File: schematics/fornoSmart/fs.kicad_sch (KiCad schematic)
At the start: 7 parts, among them J1 display, J2 rtc, J3-B rele, J4 speaker, J5 led, J6 VIN-12V

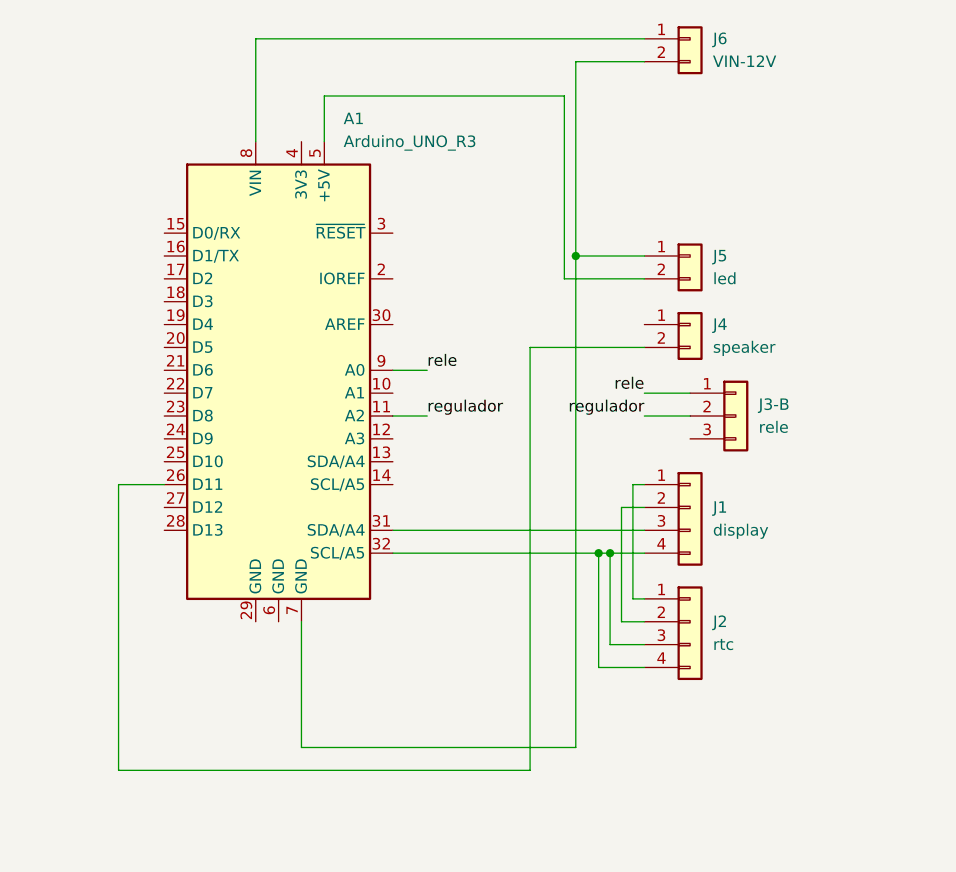
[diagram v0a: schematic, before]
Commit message: 2025-12 update
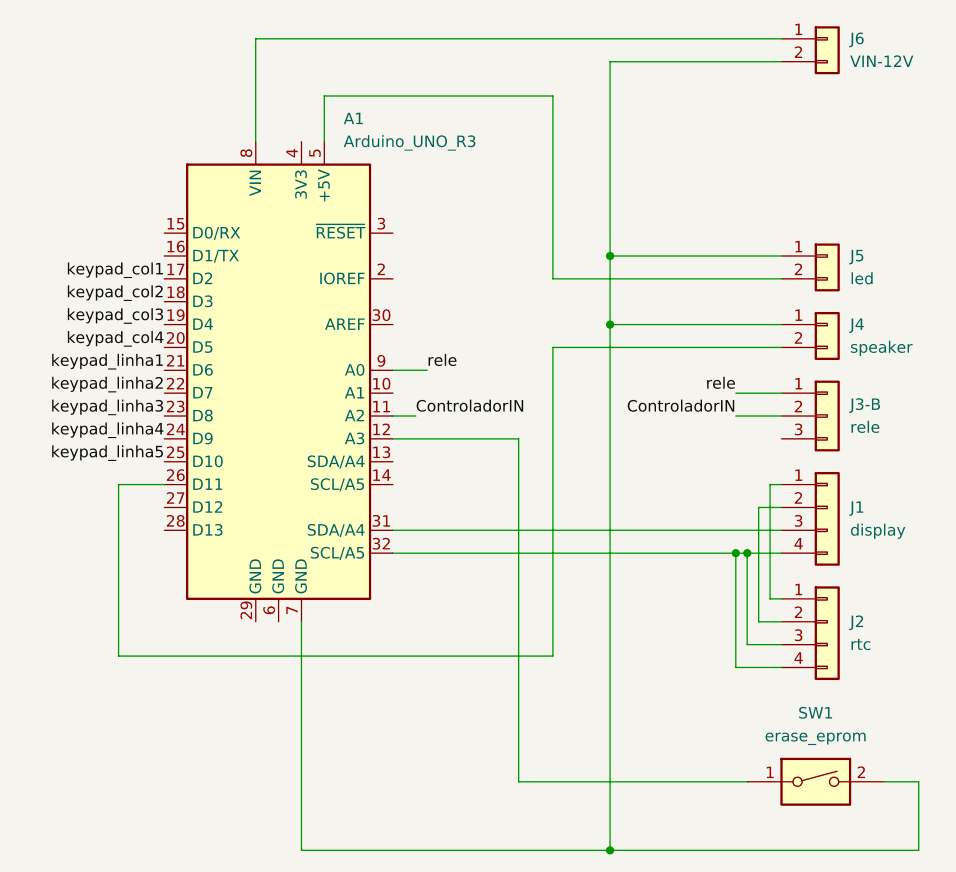
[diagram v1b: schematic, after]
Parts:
- added SW1: erase_eprom, symbol Switch:SW_DIP_x01
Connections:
- net at J4.1 (Pin_1): now also A1.7 (GND), J5.1 (Pin_1), J6.2 (Pin_2), SW1.2
- net at A1.12 (A3): now also SW1.1
- net keypad_col1: now reaches A1.17 (D2)
- net keypad_col2: now reaches A1.18 (D3)
- net keypad_col3: now reaches A1.19 (D4)
- net keypad_col4: now reaches A1.20 (D5)
- net keypad_linha1: now reaches A1.21 (D6)
- net keypad_linha2: now reaches A1.22 (D7)
- net keypad_linha3: now reaches A1.23 (D8)
- net keypad_linha4: now reaches A1.24 (D9)
- net keypad_linha5: now reaches A1.25 (D10)
- net regulador renamed ControladorIN
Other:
- moved on the sheet: J1, J2, J3-B, J4, J5, J6
